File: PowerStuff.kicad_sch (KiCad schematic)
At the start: 28 parts, among them J23 UJC-HP-L-G-5-MSMT-TR, U12 TPS2117DRLR, U14 INA260AIPW, U17 LM3480IM3-5.0, U20 AZ1117IH-3.3TRG1

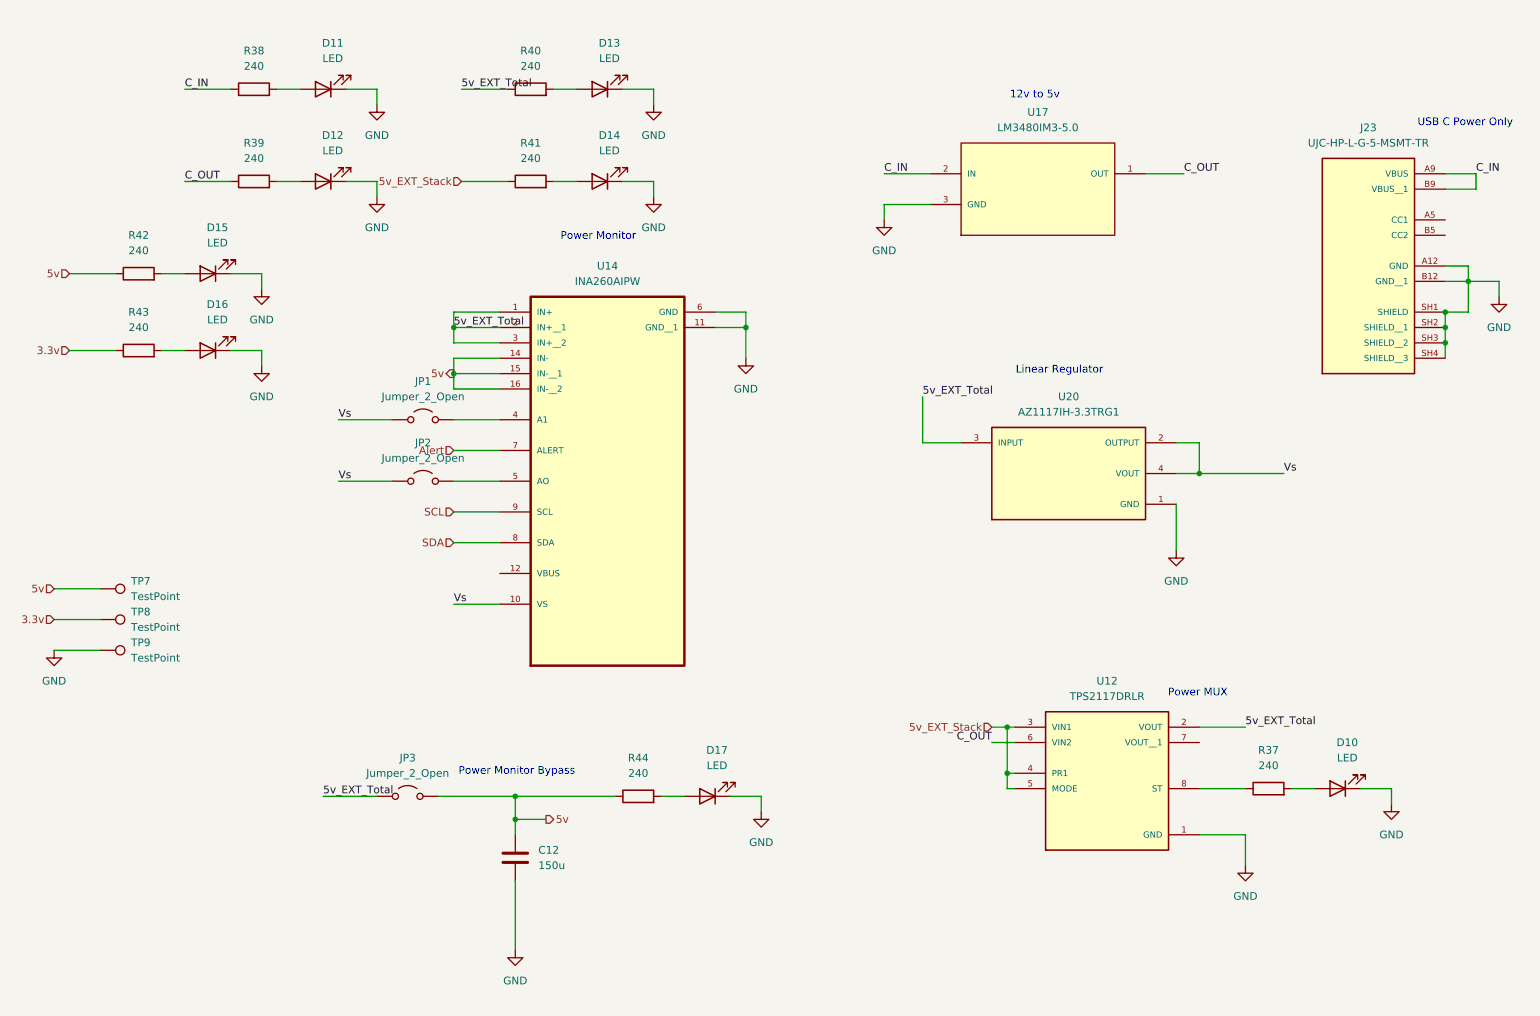
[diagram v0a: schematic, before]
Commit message: stuff
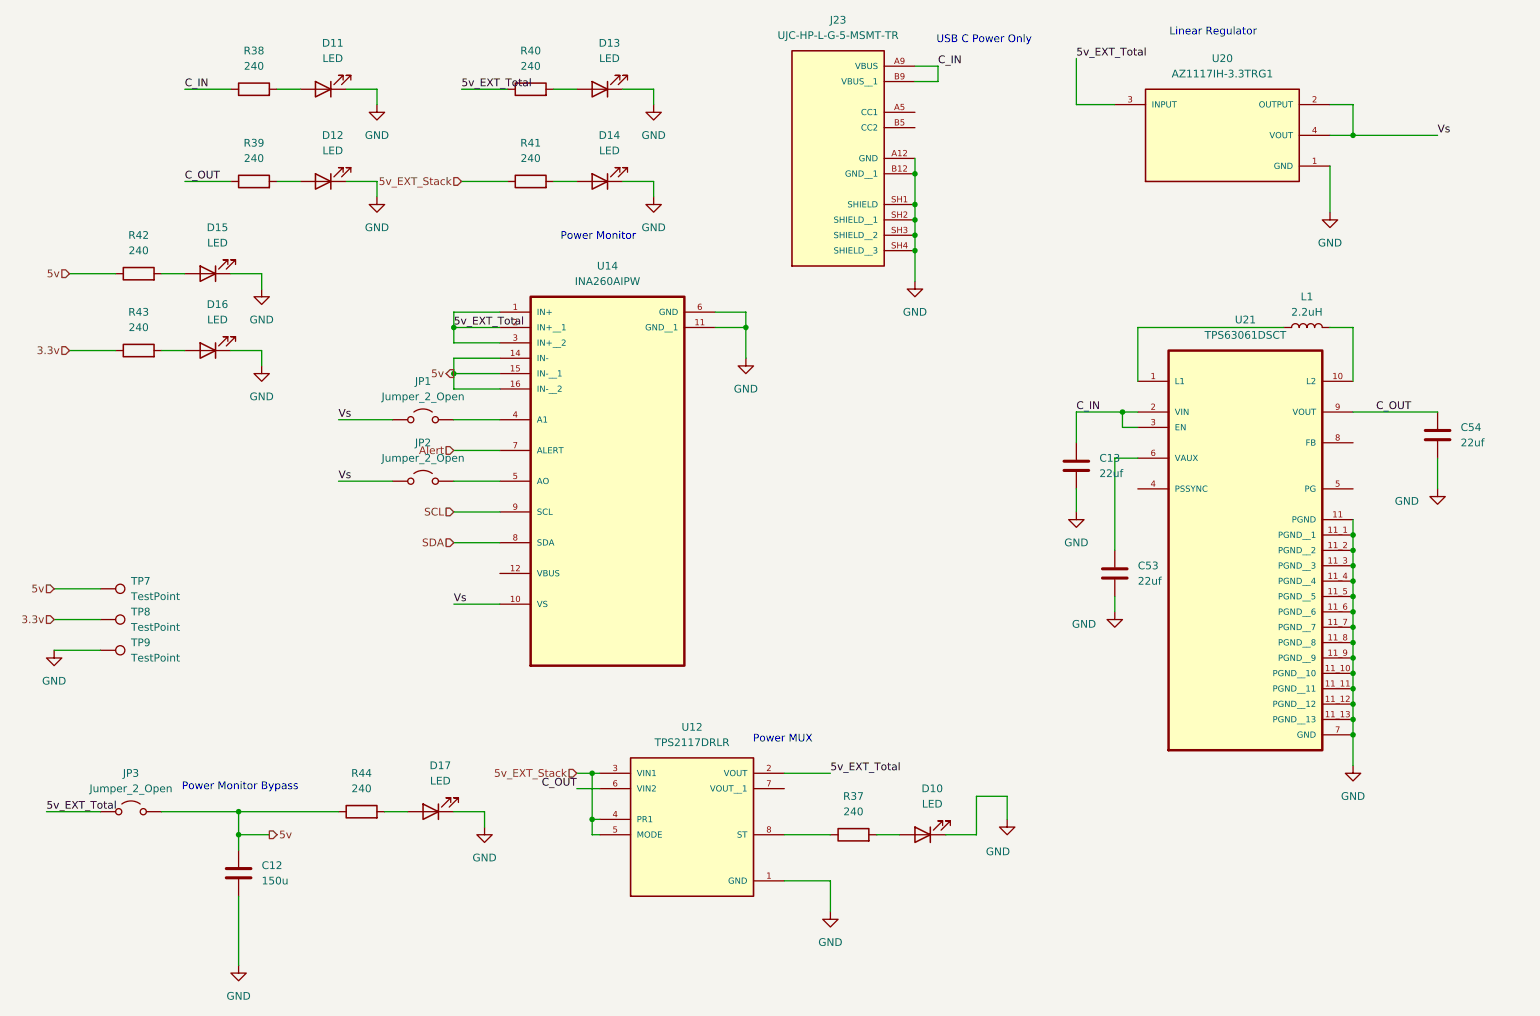
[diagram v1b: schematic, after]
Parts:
- removed U17: LM3480IM3-5.0, LM3480IM3-5.0:SOT95P263X110-3N, symbol LM3480IM3-5.0:LM3480IM3-5.0
- added C13, C53, C54: 22uf, symbol Device:C
- added L1: 2.2uH, symbol Device:L
- added U21: TPS63061DSCT, TPS63061DSCT:CONV_TPS63061DSCT, symbol TPS63061DSCT:TPS63061DSCT
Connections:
- net C_IN: now also C13.1, U21.2 (VIN), U21.3 (EN)
- net C_OUT: now also C54.1, U21.9 (VOUT)
- net GND: now also C13.2, C53.2, C54.2, U21.11 (PGND), U21.11_1 (PGND__1), U21.11_10 (PGND__10), U21.11_11 (PGND__11), U21.11_12 (PGND__12), U21.11_13 (PGND__13), U21.11_2 (PGND__2), U21.11_3 (PGND__3), U21.11_4 (PGND__4), U21.11_5 (PGND__5), U21.11_6 (PGND__6), U21.11_7 (PGND__7), U21.11_8 (PGND__8), U21.11_9 (PGND__9), U21.7 (GND)
- new net: L1.1, U21.1 (L1)
- new net: L1.2, U21.10 (L2)
- new net: C53.1, U21.6 (VAUX)
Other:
- note removed: "12v to 5v"
- moved on the sheet: C12, D10, D17, J23, JP3, R37, R44, U12, U20
